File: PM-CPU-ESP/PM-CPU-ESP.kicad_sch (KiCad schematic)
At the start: 22 parts, among them IC2 USR-ES1, J10 2EDGR-5.08-02P, J11 2EDGR-5.08-02P, J12 PinHeader P2.54 01x08 THT Ang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, J2 PinHeader P2.54 01x12 THT Str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, J3 PinHeader P2.54 01x12 THT Str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, J4 2EDGR-5.08-02P, J5 FemaleHeader P2.54 02x08 SMD 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, J9 2EDGR-5.08-02P, U3 DS3231, U4 ESP32-C3, U5 64900001039, U6 64900001039

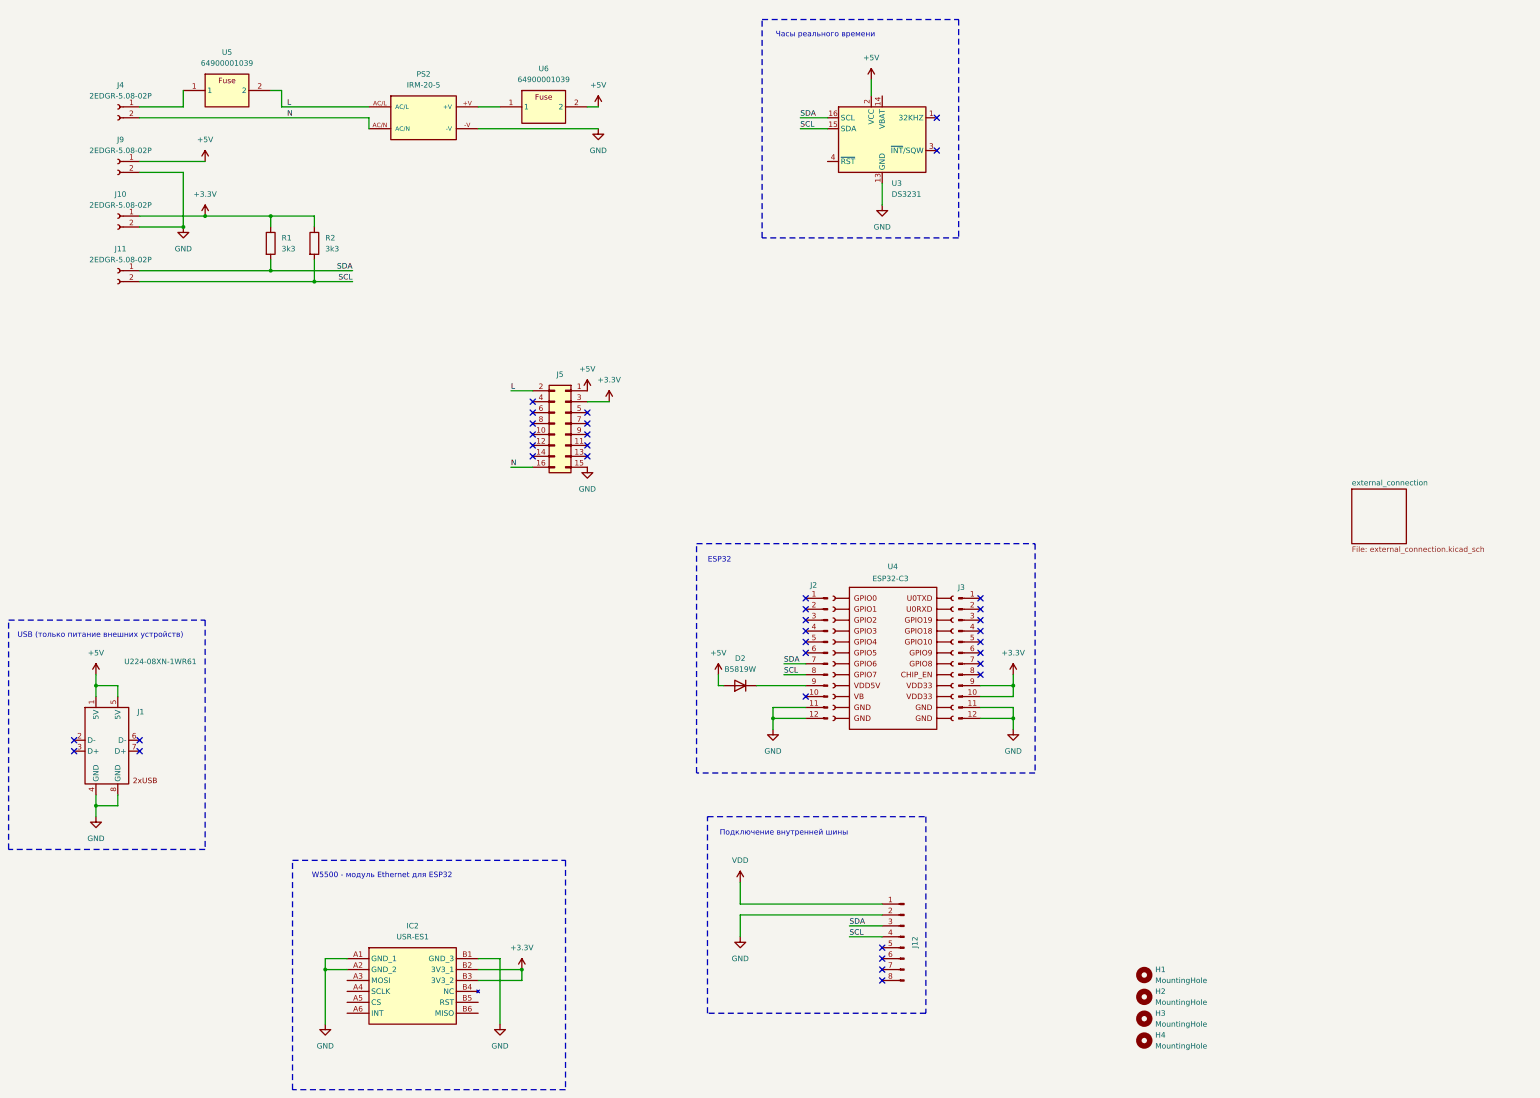
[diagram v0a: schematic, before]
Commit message: PM-CPU-ESP
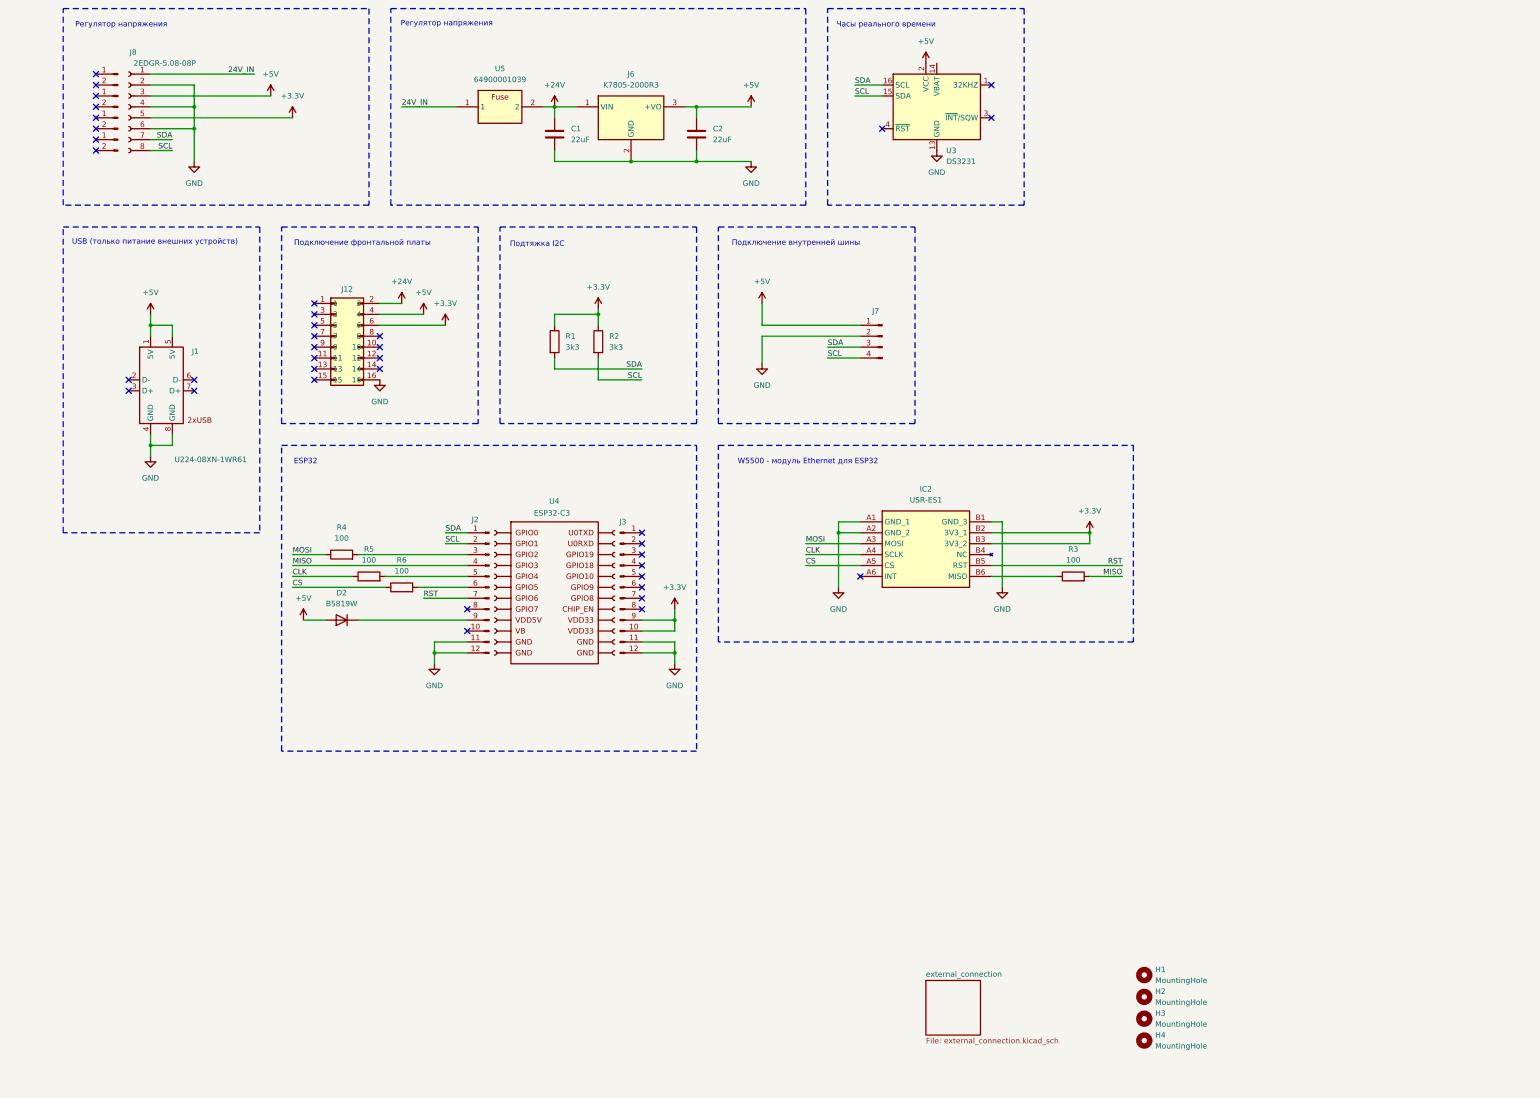
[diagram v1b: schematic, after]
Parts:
- removed J10, J11, J4, J9: 2EDGR-5.08-02P, NextPCB:Degson_2EDGR-5.08-02P, symbol NextPCB:Degson_2EDGR-5.08-02P
- removed J12: PinHeader P2.54 01x08 THT Angle, Connector_PinHeader_2.54mm:PinHeader_1x08_P2.54mm_Horizontal, symbol kicad_inventree_lib:PinHeader P2.54 01x08 THT Angle
- removed J5: FemaleHeader P2.54 02x08 SMD Straight, Connector_PinSocket_2.54mm:PinSocket_2x08_P2.54mm_Vertical_SMD, symbol kicad_inventree_lib:FemaleHeader P2.54 02x08 SMD Straight
- removed PS2: IRM-20-5, NextPCB:Meanwell-IRM-20-5, symbol kicad_inventree_lib:Meanwell-IRM-20-5
- removed U6: 64900001039, NextPCB:Fuseholder, symbol kicad_inventree_lib:Fuseholder
- added C1, C2: 22uF, kicad_inventree_lib:C_2220_5750Metric_Pad1.97x5.40mm_HandSolder, symbol kicad_inventree_lib:C_22uF_50V_2220
- added J10, J11, J4, J9: 2EDGK-5.08-02P, symbol kicad_inventree_lib:Degson_2EDGK-5.08-02P
- added J12: ~, kicad_inventree_lib:PM-front-02x08, symbol kicad_inventree_lib:PM-front-02x08
- added J6: K7805-2000R3, kicad_inventree_lib:K7805-2000R3, symbol kicad_inventree_lib:K7805-2000R3
- added J7: Conn_01x04_Pin, Connector_PinHeader_2.54mm:PinHeader_1x04_P2.54mm_Horizontal, symbol kicad_inventree_lib:PinHeader P2.54 01x04 THT Angle
- added J8: 2EDGR-5.08-08P, kicad_inventree_lib:Degson_2EDGR-5.08-08P, symbol kicad_inventree_lib:Degson_2EDGR-5.08-08P
- added R3, R4, R5, R6: 100, Resistor_SMD:R_1206_3216Metric_Pad1.30x1.75mm_HandSolder, symbol kicad_inventree_lib:R_100_1206_1%
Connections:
- net +3.3V: now also J12.6, J8.5 (Pin_5)
- net +5V: now also C2.1, J12.4, J6.3 (+VO), J7.1 (Pin_1), J8.3 (Pin_3)
- net GND: now also C1.2, C2.2, J12.16, J6.2 (GND), J7.2 (Pin_2), J8.2 (Pin_2), J8.4 (Pin_4), J8.6 (Pin_6)
- net SCL: now also J2.2 (Pin_2), J7.4 (Pin_4), J8.8 (Pin_8); no longer J2.8 (Pin_8)
- net SDA: now also J2.1 (Pin_1), J7.3 (Pin_3), J8.7 (Pin_7); no longer J2.7 (Pin_7)
- net at J2.3 (Pin_3): now also R4.2
- net MISO: now reaches J2.4 (Pin_4)
- net MISO: now also R3.2
- net at J2.5 (Pin_5): now also R5.2
- net at J2.6 (Pin_6): now also R6.2
- net 24V_IN: now reaches U5.1
- net 24V_IN: now also J8.1 (Pin_1)
- net MOSI: now reaches IC2.A3 (MOSI)
- net MOSI: now also R4.1
- net CLK: now reaches IC2.A4 (SCLK)
- net CLK: now also R5.1
- net CS: now reaches IC2.A5 (CS)
- net CS: now also R6.1
- net RST: now reaches IC2.B5 (RST)
- net RST: now also J2.7 (Pin_7)
- net at IC2.B6 (MISO): now also R3.1
- net L renamed +24V
- net +24V: now also C1.1, J12.2, J6.1 (VIN)
- no-connect marks 36 -> 38
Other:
- note added: "Подключение фронтальной платы"
- note added: "Подтяжка I2C"
- note added: "Регулятор напряжения"
- moved on the sheet: D2, IC2, J1, J2, J3, R1, R2, U3, U4, U5
